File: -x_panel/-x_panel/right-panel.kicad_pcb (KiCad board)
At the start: 2 copper layers, 85 x 270 mm, 12 parts

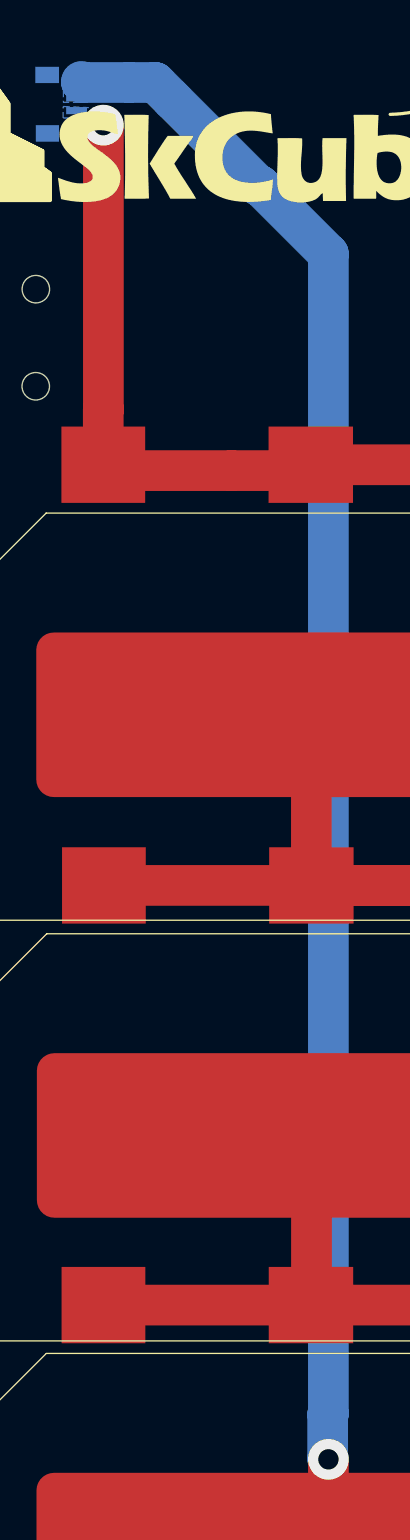
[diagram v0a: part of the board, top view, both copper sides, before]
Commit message: Rerouted some stuff
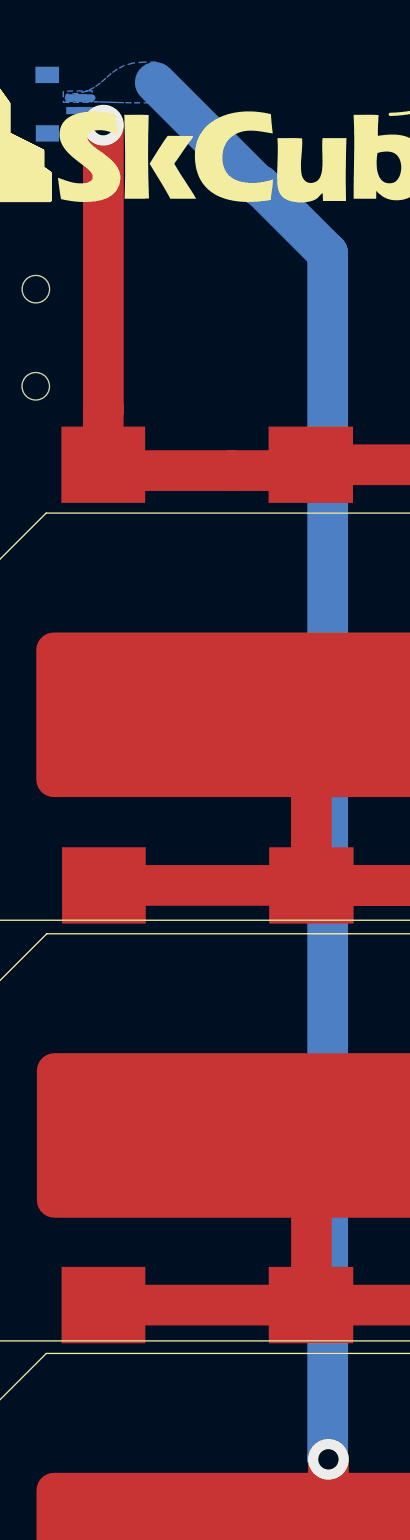
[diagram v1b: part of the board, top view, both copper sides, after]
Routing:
- net Net-(SC13--): track 159.2 -> 153.3 mm
- net Net-(SC2-+): track 88.4 -> 92.5 mm
- removed copper zone on B.Cu, net Net-(SC2-+)
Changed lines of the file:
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@@
 			(best_width_ratio 1)
 			(max_width 2)
-			(curved_edges no)
+			(curved_edges yes)
 			(filter_ratio 0.9)
 			(enabled yes)
@@
 			(prefer_zone_connections yes)
 		)
+		(net 3)
+	)
+	(segment
+		(start 954.781726 56.7175)
+		(end 957.415117 56.7175)
+		(width 0.7)
+		(layer "B.Cu")
+		(net 3)
+	)
+	(segment
+		(start 957.415117 56.7175)
+		(end 957.415117 58.15)
+		(width 0.7)
+		(layer "B.Cu")
 		(net 3)
 	)
@@
 	)
 	(segment
-		(start 979.45 189.15)
-		(end 979.45 184.82)
-		(width 4)
-		(layer "B.Cu")
-		(net 4)
-	)
-	(segment
 		(start 972.790111 64.069)
 		(end 972.629 64.069)
-		(width 4)
-		(layer "B.Cu")
-		(net 4)
-	)
-	(segment
-		(start 955.257726 53.93)
-		(end 955.257726 53.85)
 		(width 4)
 		(layer "B.Cu")
@@
 	(segment
 		(start 972.629 64.069)
-		(end 964.2 55.64)
-		(width 4)
-		(layer "B.Cu")
-		(net 4)
-	)
-	(segment
-		(start 959.94 53.95)
-		(end 955.277726 53.95)
-		(width 4)
-		(layer "B.Cu")
-		(net 4)
-	)
-	(segment
-		(start 964.2 55.64)
 		(end 962.51 53.95)
 		(width 4)
@@
 	)
 	(segment
-		(start 979.52 70.798889)
+		(start 979.45 70.728889)
 		(end 972.790111 64.069)
 		(width 4)
@@
 	)
 	(segment
-		(start 979.52 184.75)
-		(end 979.52 70.798889)
-		(width 4)
+		(start 954.781726 55.4625)
+		(end 956.2875 55.4625)
+		(width 0.7)
 		(layer "B.Cu")
 		(net 4)
 	)
 	(segment
-		(start 979.45 184.82)
-		(end 979.52 184.75)
-		(width 4)
-		(layer "B.Cu")
-		(net 4)
-	)
-	(segment
-		(start 962.51 53.95)
-		(end 959.94 53.95)
+		(start 979.45 189.15)
+		(end 979.45 70.728889)
 		(width 4)
 		(layer "B.Cu")
@@
 	)
 	(zone
-		(net 3)
-		(net_name "Net-(SC2-+)")
+		(net 4)
+		(net_name "Net-(SC13--)")
 		(layer "B.Cu")
 		(hatch edge 0.5)
-		(connect_pads
+		(priority 17540)
+		(connect_pads yes
 			(clearance 0)
 		)
-		(min_thickness 0.25)
+		(min_thickness 0.0254)
 		(filled_areas_thickness no)
 		(fill yes
@@
 		(polygon
 			(pts
-				(xy 953.52 56.32) (xy 957.87 56.51) (xy 958.81 59.53) (xy 955.97 57.46) (xy 953.46 57.45) (xy 953.46 56.32)
+				(xy 961.46497 51.95) (xy 960.361099 52.03855) (xy 959.485409 52.2789) (xy 958.780854 52.633099)
+				(xy 958.190389 53.0632) (xy 957.65697 53.53125) (xy 957.123551 53.9993) (xy 956.533086 54.4294)
+				(xy 955.828531 54.7836) (xy 954.952841 55.02395) (xy 953.848971 55.1125) (xy 953.796471 55.1125)
+				(xy 953.673971 55.4625) (xy 953.796471 55.8125) (xy 953.848971 55.8125) (xy 954.88488 55.81635)
+				(xy 955.737917 55.8268) (xy 956.453799 55.842199) (xy 957.078243 55.8609) (xy 957.65697 55.88125)
+				(xy 958.235697 55.9016) (xy 958.860141 55.9203) (xy 959.576023 55.9357) (xy 960.42906 55.94615)
+				(xy 961.46497 55.95) (xy 963.46497 55.95) (xy 963.76147 53.95) (xy 962.6 51.95)
 			)
 		)
+	)
+	(zone
+		(net 3)
+		(net_name "Net-(SC2-+)")
+		(layer "B.Cu")
+		(name "$teardrop_padvia$")
+		(hatch none 0.1)
+		(priority 30000)
+		(attr
+			(teardrop
+				(type padvia)
+			)
+		)
+		(connect_pads yes
+			(clearance 0)
+		)
+		(min_thickness 0.0254)
+		(filled_areas_thickness no)
+		(fill yes
+			(thermal_gap 0.5)
+			(thermal_bridge_width 0.5)
+			(island_removal_mode 1)
+			(island_area_min 10)
+		)
+		(polygon
+			(pts
+				(xy 955.043387 57.0675) (xy 955.114363 57.072371) (xy 955.17706 57.086464) (xy 955.230974 57.108497)
+				(xy 955.277841 57.137922) (xy 955.35457 57.219392) (xy 955.411325 57.335228) (xy 955.447262 57.493921)
+				(xy 955.458513 57.704514) (xy 955.441381 57.990648) (xy 955.432227 58.120372) (xy 957.416117 58.15)
+				(xy 956.466054 56.408297) (xy 956.356636 56.446249) (xy 956.200359 56.458372) (xy 955.948522 56.439863)
+				(xy 955.812834 56.423957) (xy 955.459944 56.38608) (xy 955.043387 56.3675)
+			)
+		)
